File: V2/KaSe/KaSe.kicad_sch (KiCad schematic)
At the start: 159 parts, among them J1 gc9a01_DISPLAY, J2 Conn_01x06, J3 Conn_01x04_Pin, J4 Conn_01x03, J5 Conn_01x03, Q1 BSS83P, Q2 BSS83P, SW1 SWITCH_PUSH, SW10 SWITCH_PUSH, SW11 SWITCH_PUSH, SW12 SWITCH_PUSH, SW13 SWITCH_PUSH, SW14 SWITCH_PUSH, SW15 SWITCH_PUSH, SW16 SWITCH_PUSH, SW17 SWITCH_PUSH, SW18 SWITCH_PUSH, SW19 SWITCH_PUSH, SW2 SWITCH_PUSH, SW20 SWITCH_PUSH, SW21 SWITCH_PUSH, SW22 SWITCH_PUSH, SW23 SWITCH_PUSH, SW24 SWITCH_PUSH, SW25 SWITCH_PUSH, SW26 SWITCH_PUSH, SW27 SWITCH_PUSH, SW28 SWITCH_PUSH, SW29 SWITCH_PUSH, SW3 SWITCH_PUSH, SW30 SWITCH_PUSH, SW31 SWITCH_PUSH, SW32 SWITCH_PUSH, SW33 SWITCH_PUSH, SW34 SWITCH_PUSH, SW36 SWITCH_PUSH, SW37 SWITCH_PUSH, SW38 SWITCH_PUSH, SW39 SWITCH_PUSH, SW4 SWITCH_PUSH, SW40 SWITCH_PUSH, SW41 SWITCH_PUSH, SW42 SWITCH_PUSH, SW43 SWITCH_PUSH, SW44 SWITCH_PUSH, SW45 SWITCH_PUSH, SW46 SWITCH_PUSH, SW47 SWITCH_PUSH, SW48 SWITCH_PUSH, SW49 SWITCH_PUSH, SW5 SWITCH_PUSH, SW50 SWITCH_PUSH, SW51 SWITCH_PUSH, SW52 SWITCH_PUSH, SW53 SWITCH_PUSH, SW54 SWITCH_PUSH, SW55 SWITCH_PUSH, SW56 SWITCH_PUSH, SW57 SWITCH_PUSH, SW58 SWITCH_PUSH, SW59 SWITCH_PUSH, SW6 SWITCH_PUSH, SW60 SWITCH_PUSH, SW61 SWITCH_PUSH, SW62 SWITCH_PUSH, SW63 SWITCH_PUSH, SW64 SWITCH_PUSH, SW65 SWITCH_PUSH, SW7 SWITCH_PUSH, SW8 SWITCH_PUSH, SW9 SWITCH_PUSH, U1 NRF24L01_Breakout, U2 AP130-33SA, U3 ESP32-S3-DevKitC, U4 TLV73333PDBV

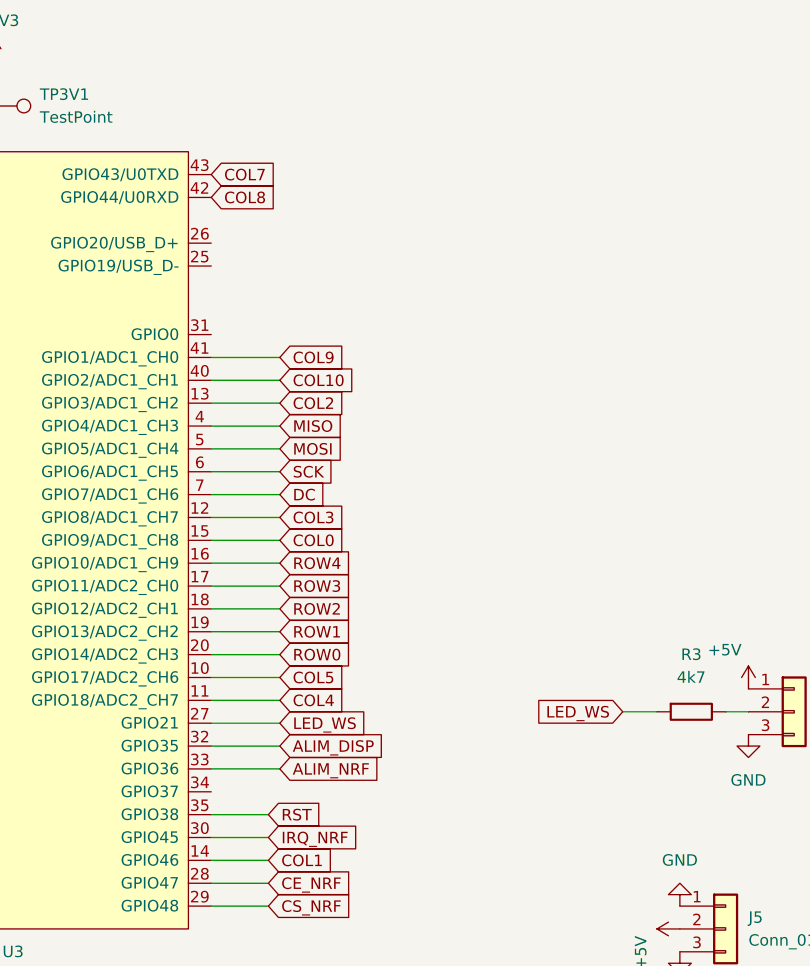
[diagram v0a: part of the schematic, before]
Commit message: e
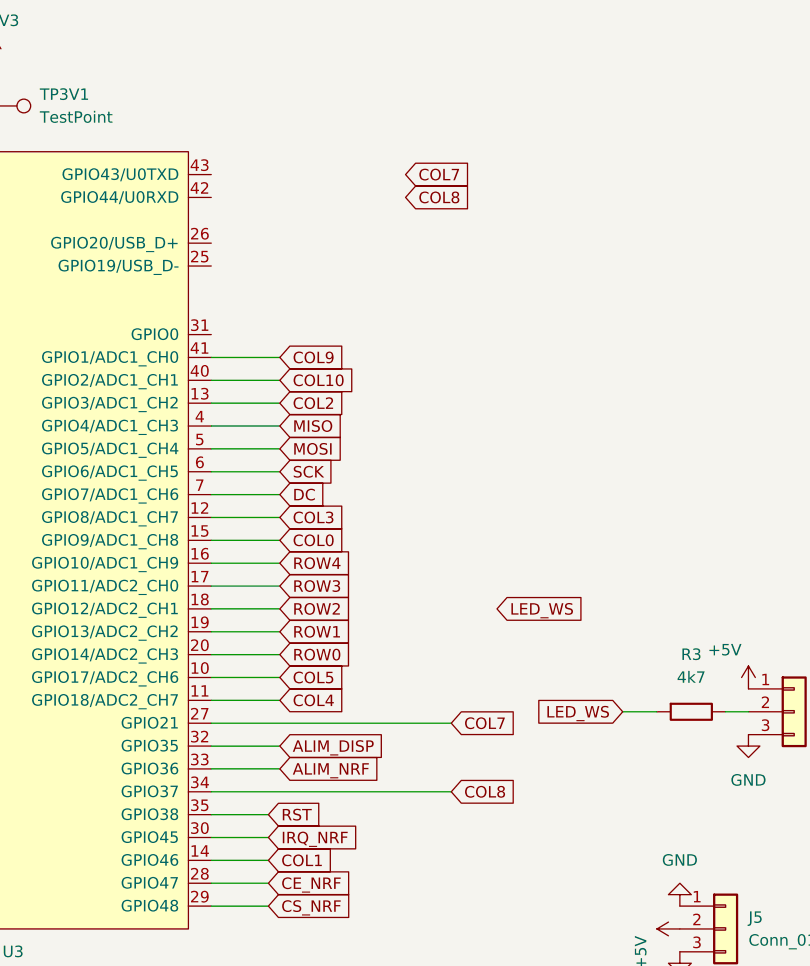
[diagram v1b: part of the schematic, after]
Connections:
- net COL7: now also U3.27 (GPIO21); no longer U3.43 (GPIO43/U0TXD)
- net COL8: now also U3.34 (GPIO37); no longer U3.42 (GPIO44/U0RXD)
- net LED_WS: no longer U3.27 (GPIO21)
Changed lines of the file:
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@@
 	(wire
 		(pts
-			(xy 488.95 124.46) (xy 481.33 124.46)
-		)
-		(stroke
-			(width 0)
-			(type default)
-		)
-	)
-	(wire
-		(pts
 			(xy 335.28 130.81) (xy 335.28 125.73)
 		)
@@
 	(wire
 		(pts
+			(xy 508 132.08) (xy 481.33 132.08)
+		)
+		(stroke
+			(width 0)
+			(type default)
+		)
+	)
+	(wire
+		(pts
 			(xy 488.95 91.44) (xy 481.33 91.44)
 		)
@@
 	(wire
 		(pts
+			(xy 481.33 124.46) (xy 508 124.46)
+		)
+		(stroke
+			(width 0)
+			(type default)
+		)
+	)
+	(wire
+		(pts
 			(xy 86.36 77.47) (xy 86.36 85.09)
 		)
@@
 		)
 	)
+	(global_label "COL8"
+		(shape input)
+		(at 502.92 66.04 0)
+		(fields_autoplaced yes)
+		(effects
+			(font
+				(size 1.27 1.27)
+			)
+			(justify left)
+		)
+		(property "Intersheetrefs" "${INTERSHEET_REFS}"
+			(at 510.0891 66.04 0)
+			(effects
+				(font
+					(size 1.27 1.27)
+				)
+				(justify left)
+				(hide yes)
+			)
+		)
+	)
 	(global_label "ALIM_DISP"
 		(shape input)
@@
 		)
 	)
+	(global_label "COL7"
+		(shape input)
+		(at 502.92 63.5 0)
+		(fields_autoplaced yes)
+		(effects
+			(font
+				(size 1.27 1.27)
+			)
+			(justify left)
+		)
+		(property "Intersheetrefs" "${INTERSHEET_REFS}"
+			(at 510.0891 63.5 0)
+			(effects
+				(font
+					(size 1.27 1.27)
+				)
+				(justify left)
+				(hide yes)
+			)
+		)
+	)
 	(global_label "OUT+"
 		(shape input)
@@
 	(global_label "COL8"
 		(shape input)
-		(at 481.33 66.04 0)
+		(at 508 132.08 0)
 		(fields_autoplaced yes)
 		(effects
@@
 		)
 		(property "Intersheetrefs" "${INTERSHEET_REFS}"
-			(at 488.4991 66.04 0)
+			(at 515.1691 132.08 0)
 			(effects
 				(font
@@
 	(global_label "LED_WS"
 		(shape input)
-		(at 488.95 124.46 0)
+		(at 513.08 111.76 0)
 		(fields_autoplaced yes)
 		(effects
@@
 		)
 		(property "Intersheetrefs" "${INTERSHEET_REFS}"
-			(at 498.3566 124.46 0)
+			(at 522.4866 111.76 0)
 			(effects
 				(font
@@
 	(global_label "COL7"
 		(shape input)
-		(at 481.33 63.5 0)
+		(at 508 124.46 0)
 		(fields_autoplaced yes)
 		(effects
@@
 		)
 		(property "Intersheetrefs" "${INTERSHEET_REFS}"
-			(at 488.4991 63.5 0)
+			(at 515.1691 124.46 0)
 			(effects
 				(font
